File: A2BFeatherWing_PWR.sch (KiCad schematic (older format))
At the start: 10 parts, among them U301 LT1930A

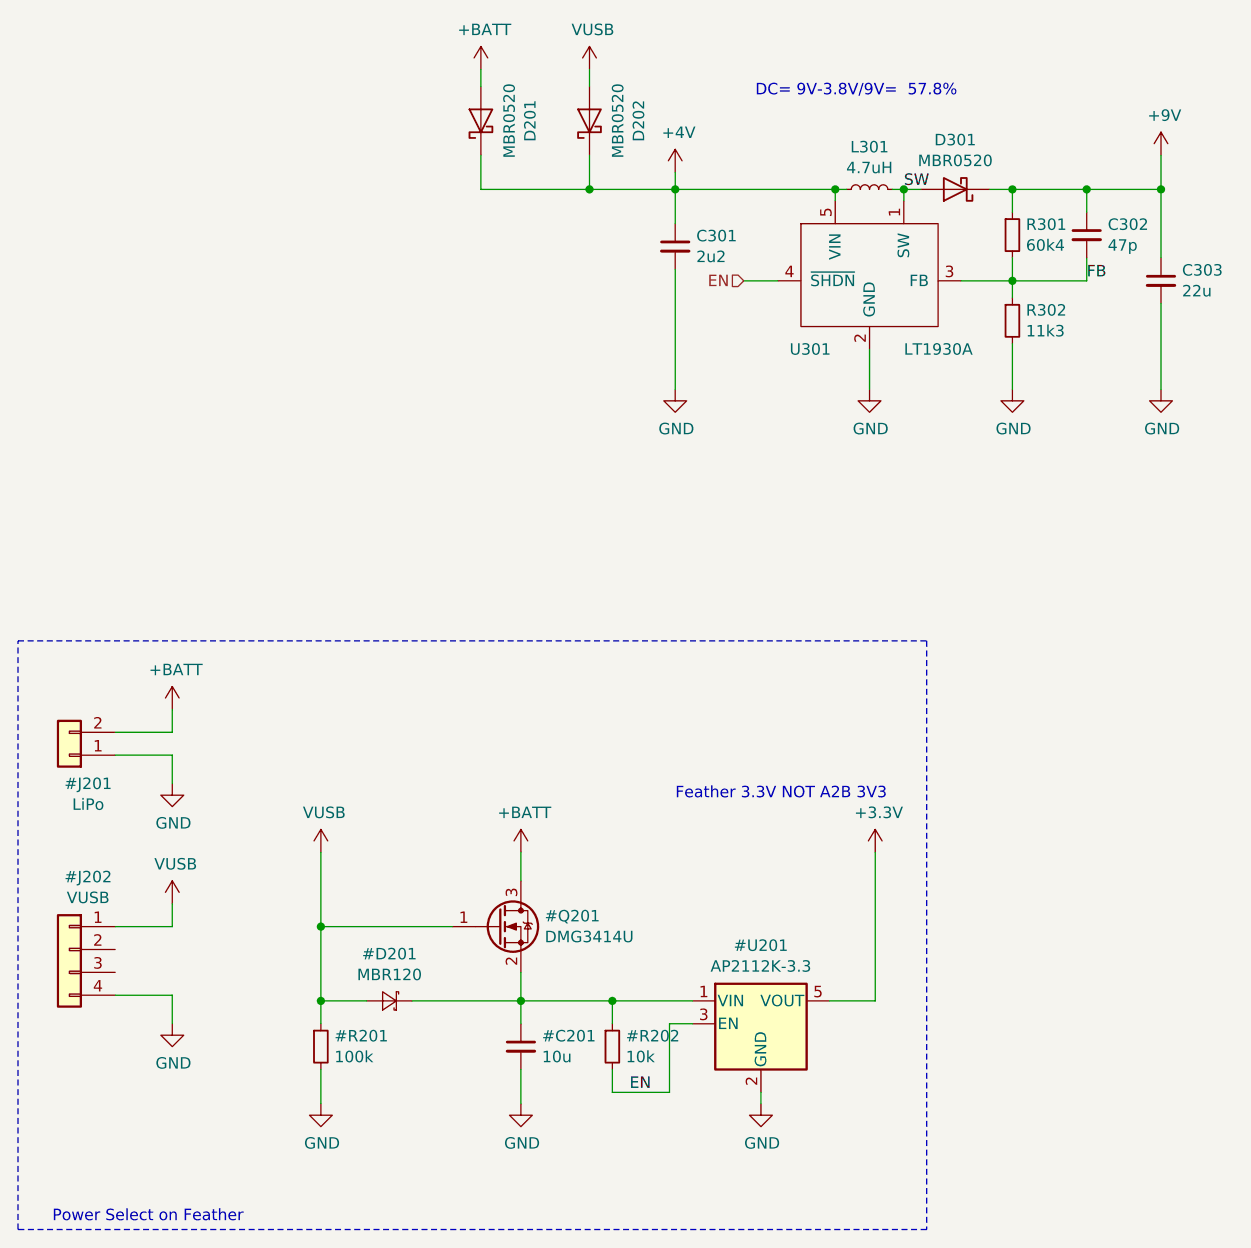
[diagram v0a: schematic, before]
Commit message: last changes
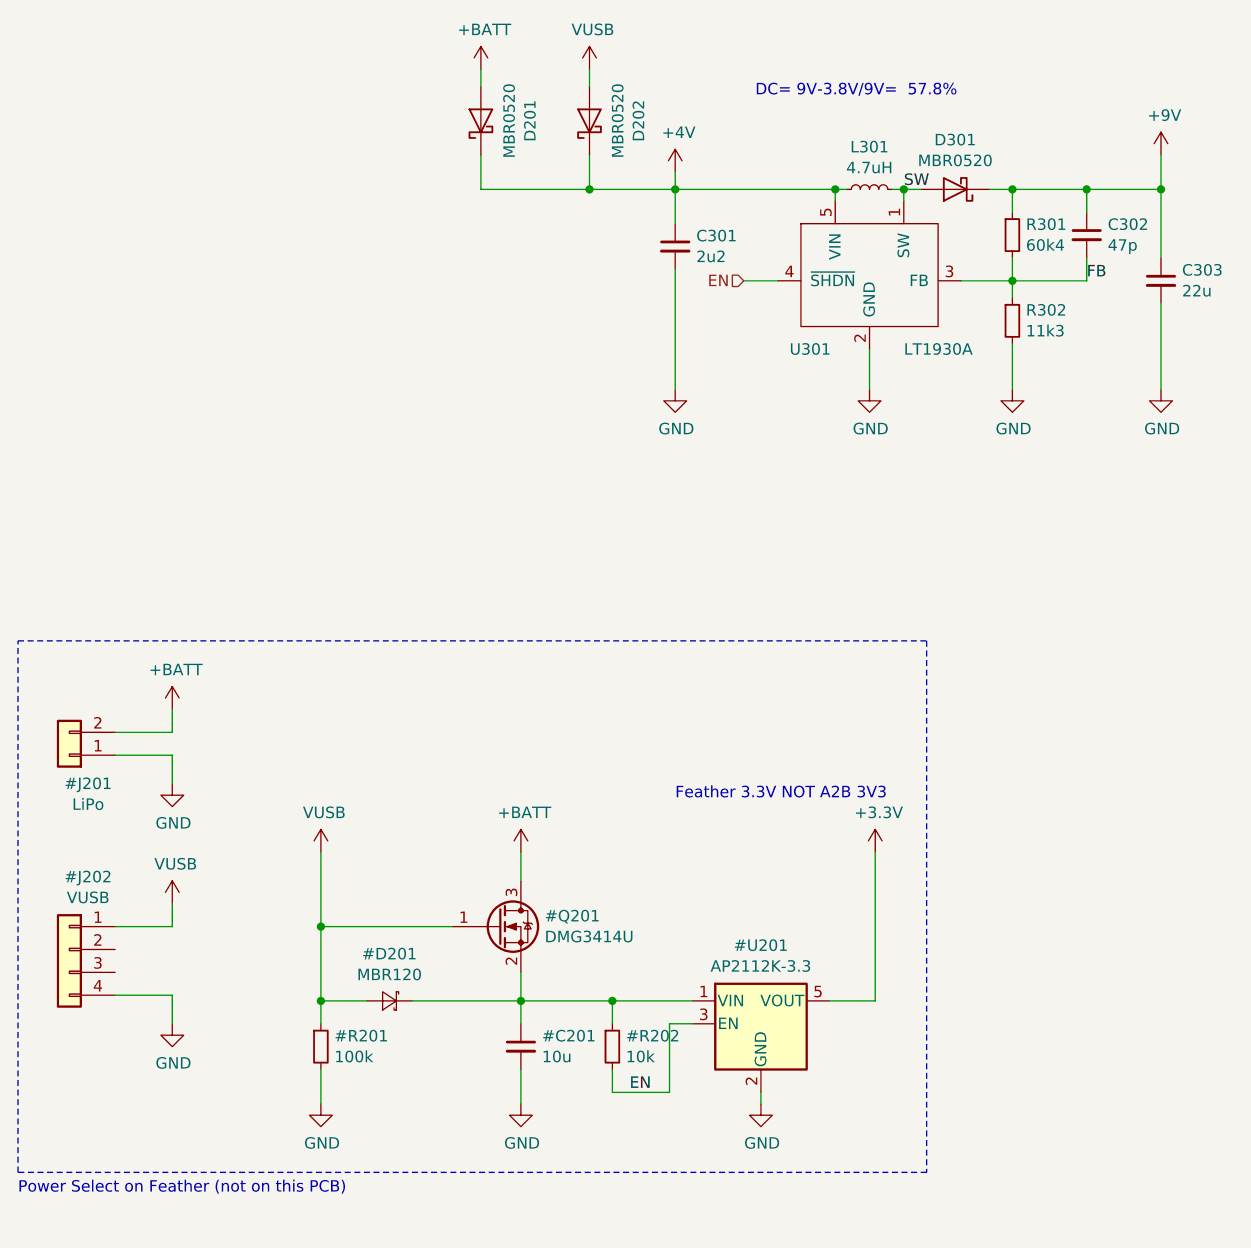
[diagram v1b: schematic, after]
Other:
- note added: "Power Select on Feather (not on this PCB)\n"
- note removed: "Power Select on Feather"
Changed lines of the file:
@@
 	850  4775 4825 4775
 Wire Notes Line
-	4825 4775 4825 7350
+	4825 4775 4825 7100
 Wire Notes Line
-	4825 7350 850  7350
+	4825 7100 850  7100
 Wire Notes Line
-	850  7350 850  4775
-Text Notes 1000 7325 0    50   ~ 0
-Power Select on Feather
+	850  7100 850  4775
+Text Notes 850  7200 0    50   ~ 0
+Power Select on Feather (not on this PCB)\n
 Wire Wire Line
 	3350 2275 3350 2350
